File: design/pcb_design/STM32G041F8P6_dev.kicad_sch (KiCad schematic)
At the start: 33 parts, among them J1 USB_B_Micro, J2 Conn_02x02_Odd_Even, J3 S2B-PH-K-S, J4 Conn_ST_STDC14, SW1 Reset, SW2 Reset, U1 MIC5301-3.3YD5, U2 STM32G041F8Px, U3 MCP73831-2-OT, U4 ADXL343BCCZ, Y1 Crystal

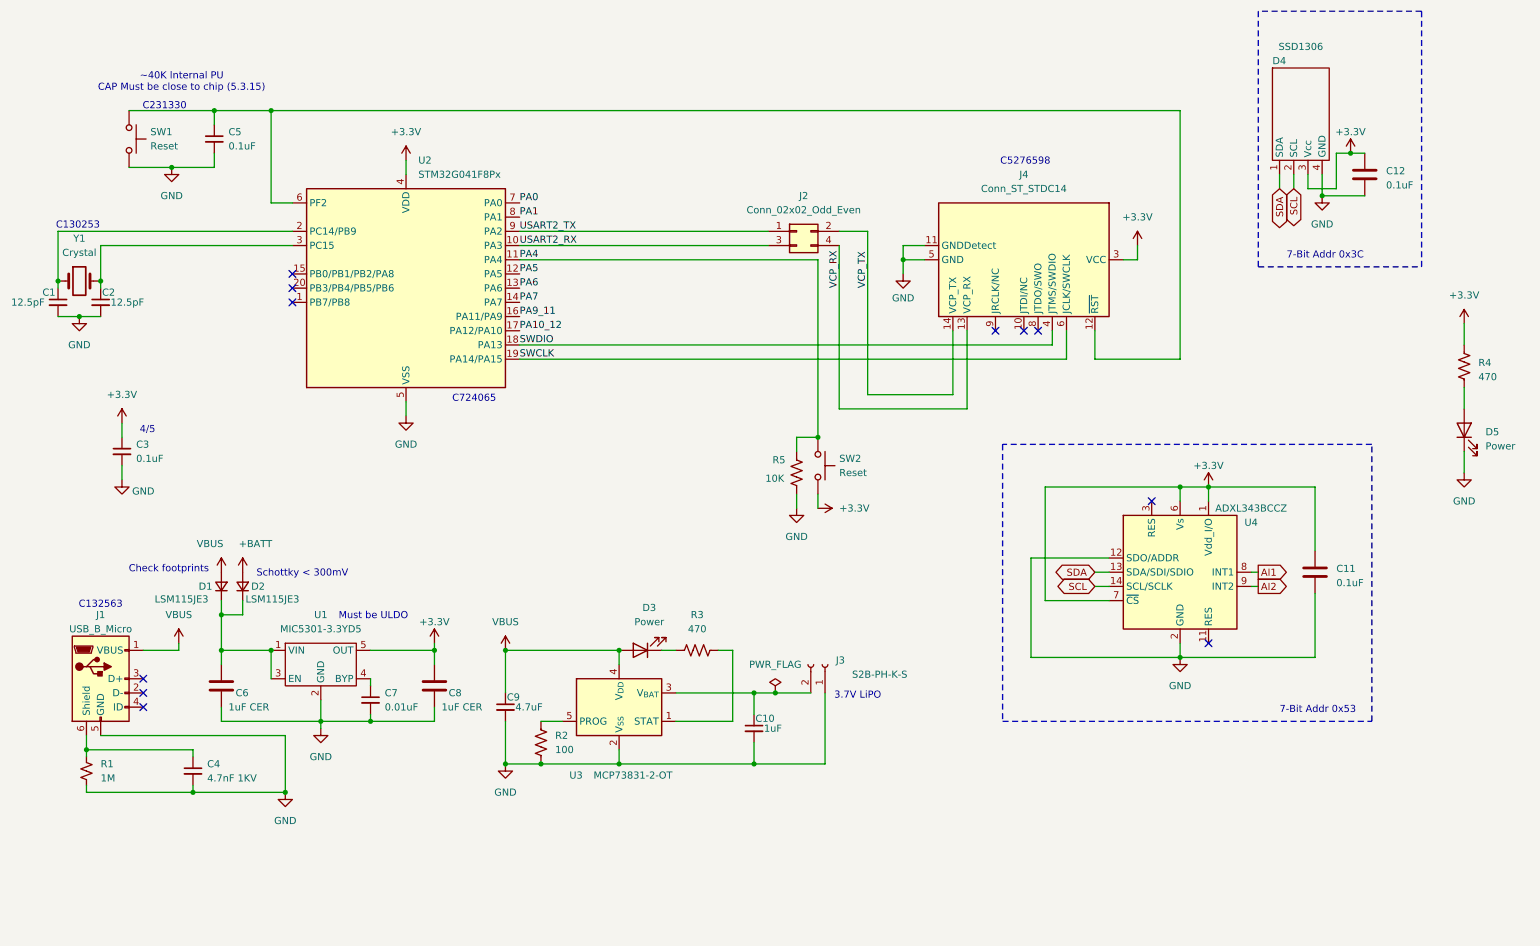
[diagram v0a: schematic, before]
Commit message: updates!
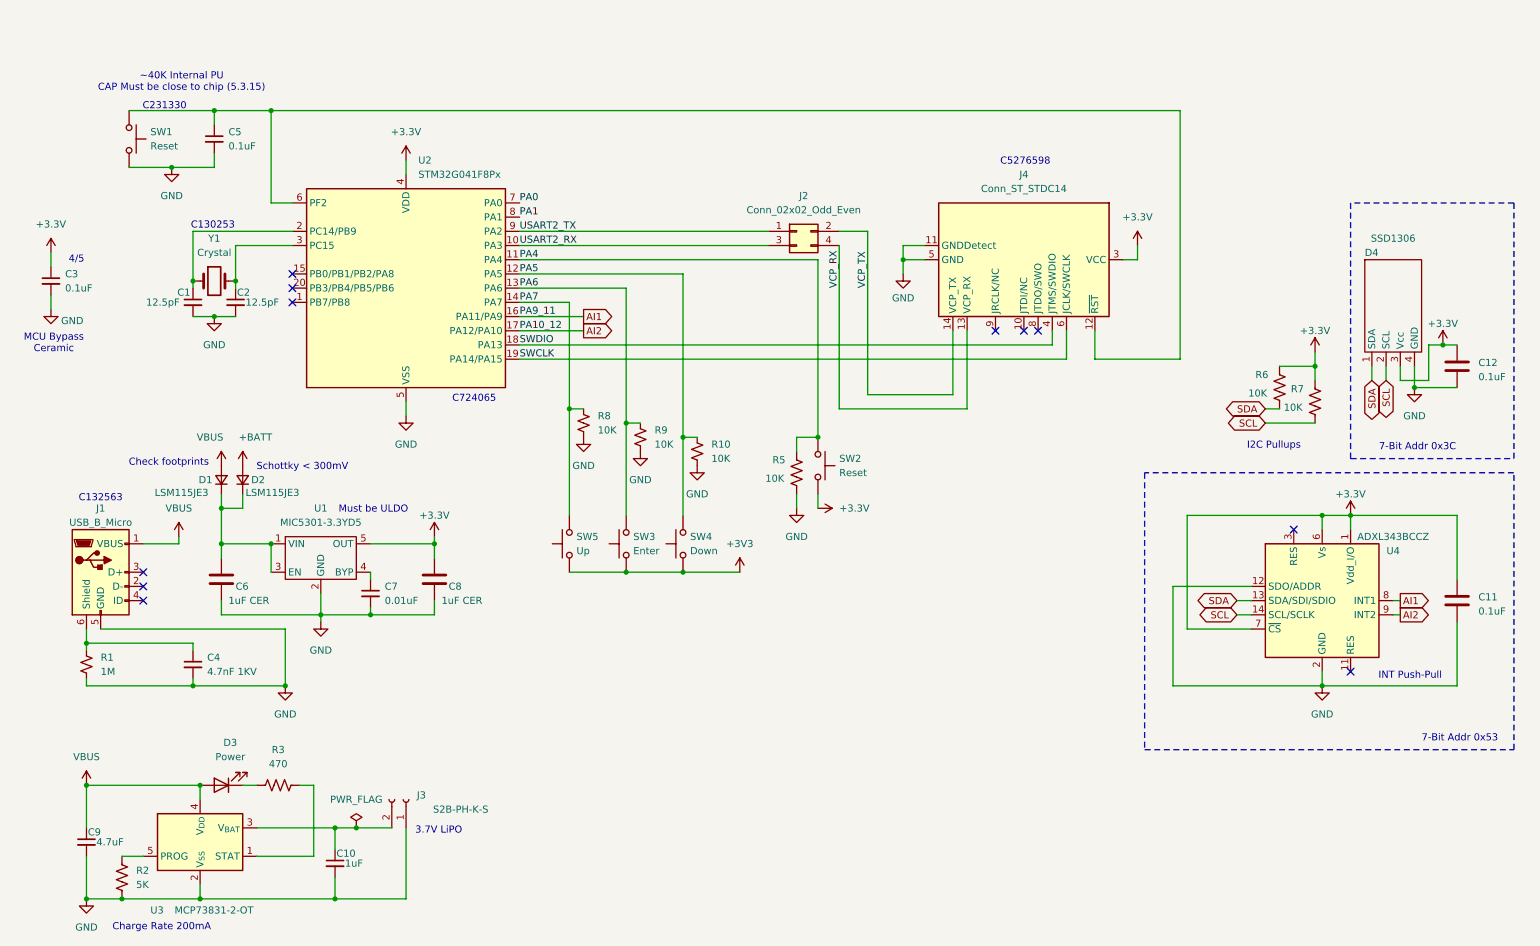
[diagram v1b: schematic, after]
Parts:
- removed D5: Power, LED_SMD:LED_0805_2012Metric, symbol Device:LED
- removed R4: 470, Resistor_SMD:R_0805_2012Metric, symbol Device:R_US
- added R10, R8, R9: 10K, symbol Device:R_Small_US
- added R6, R7: 10K, Resistor_SMD:R_0805_2012Metric, symbol Device:R_US
- added SW3: Enter, symbol Switch:SW_Push
- added SW4: Down, symbol Switch:SW_Push
- added SW5: Up, symbol Switch:SW_Push
- R2: value 100 -> 5K
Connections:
- net PA10_12 is gone; now on net AI2: U2.17 (PA12/PA10)
- net PA9_11 is gone; now on net AI1: U2.16 (PA11/PA9)
- net +3.3V: now also R6.2, R7.2
- net GND: now also R10.1, R8.1, R9.1
- net PA5: now also R10.2, SW4.2
- net PA6: now also R9.2, SW3.2
- net PA7: now also R8.2, SW5.2
- net SCL: now also R7.1
- net SDA: now also R6.1
- new net +3V3: SW3.1, SW4.1, SW5.1
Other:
- note added: "Charge Rate 200mA"
- note added: "I2C Pullups"
- note added: "INT Push-Pull"
- note added: "MCU Bypass Ceramic"
- moved on the sheet: C1, C10, C11, C12, C2, C3, C4, C6, C7, C8, C9, D1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
